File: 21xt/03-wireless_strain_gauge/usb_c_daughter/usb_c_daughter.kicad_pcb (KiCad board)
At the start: 2 copper layers, 8 x 17 mm, 3 parts, among them J1 USB_C_Plug_USB2.0, J3 Conn_01x03

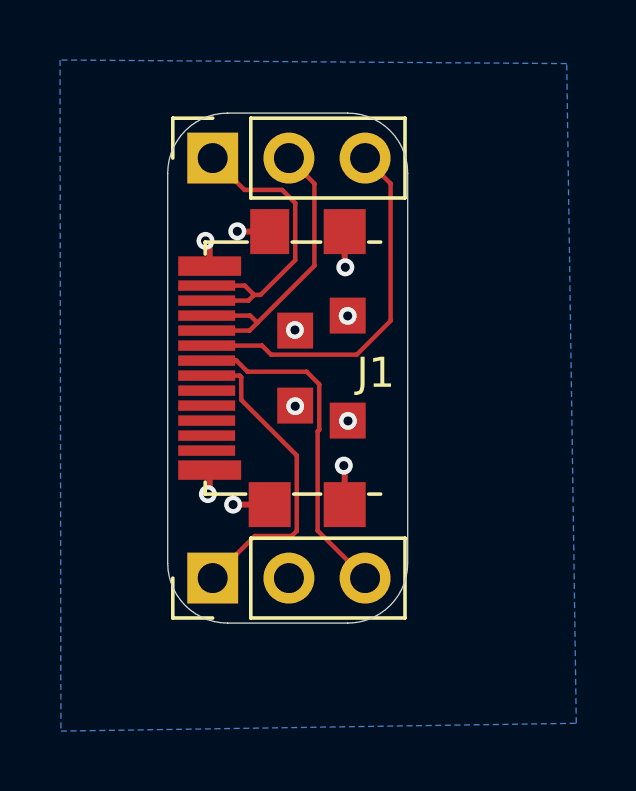
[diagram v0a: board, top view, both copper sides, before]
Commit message: v2
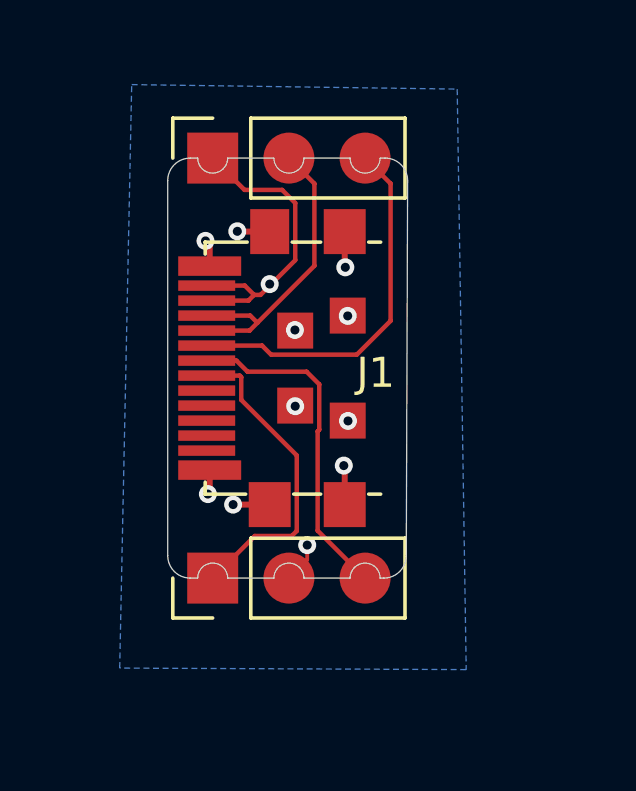
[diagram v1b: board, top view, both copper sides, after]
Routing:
- net SHIELD: track 6.61 -> 7.41 mm, vias 10 -> 11
- net GND: vias 0 -> 1
- added copper zone on In1.Cu, net GND
- added copper zone on In2.Cu, net GND
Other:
- board size 8 x 17 mm -> 8 x 14 mm
- copper layers 2 -> 4
